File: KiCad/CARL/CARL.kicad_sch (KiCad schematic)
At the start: 39 parts, among them J1 Barrel_Jack (5V DC Supply), J2 SD_Card_Device, U1 NHD-0420H1Z (LCD), U2 LM386, U3 Led Driver

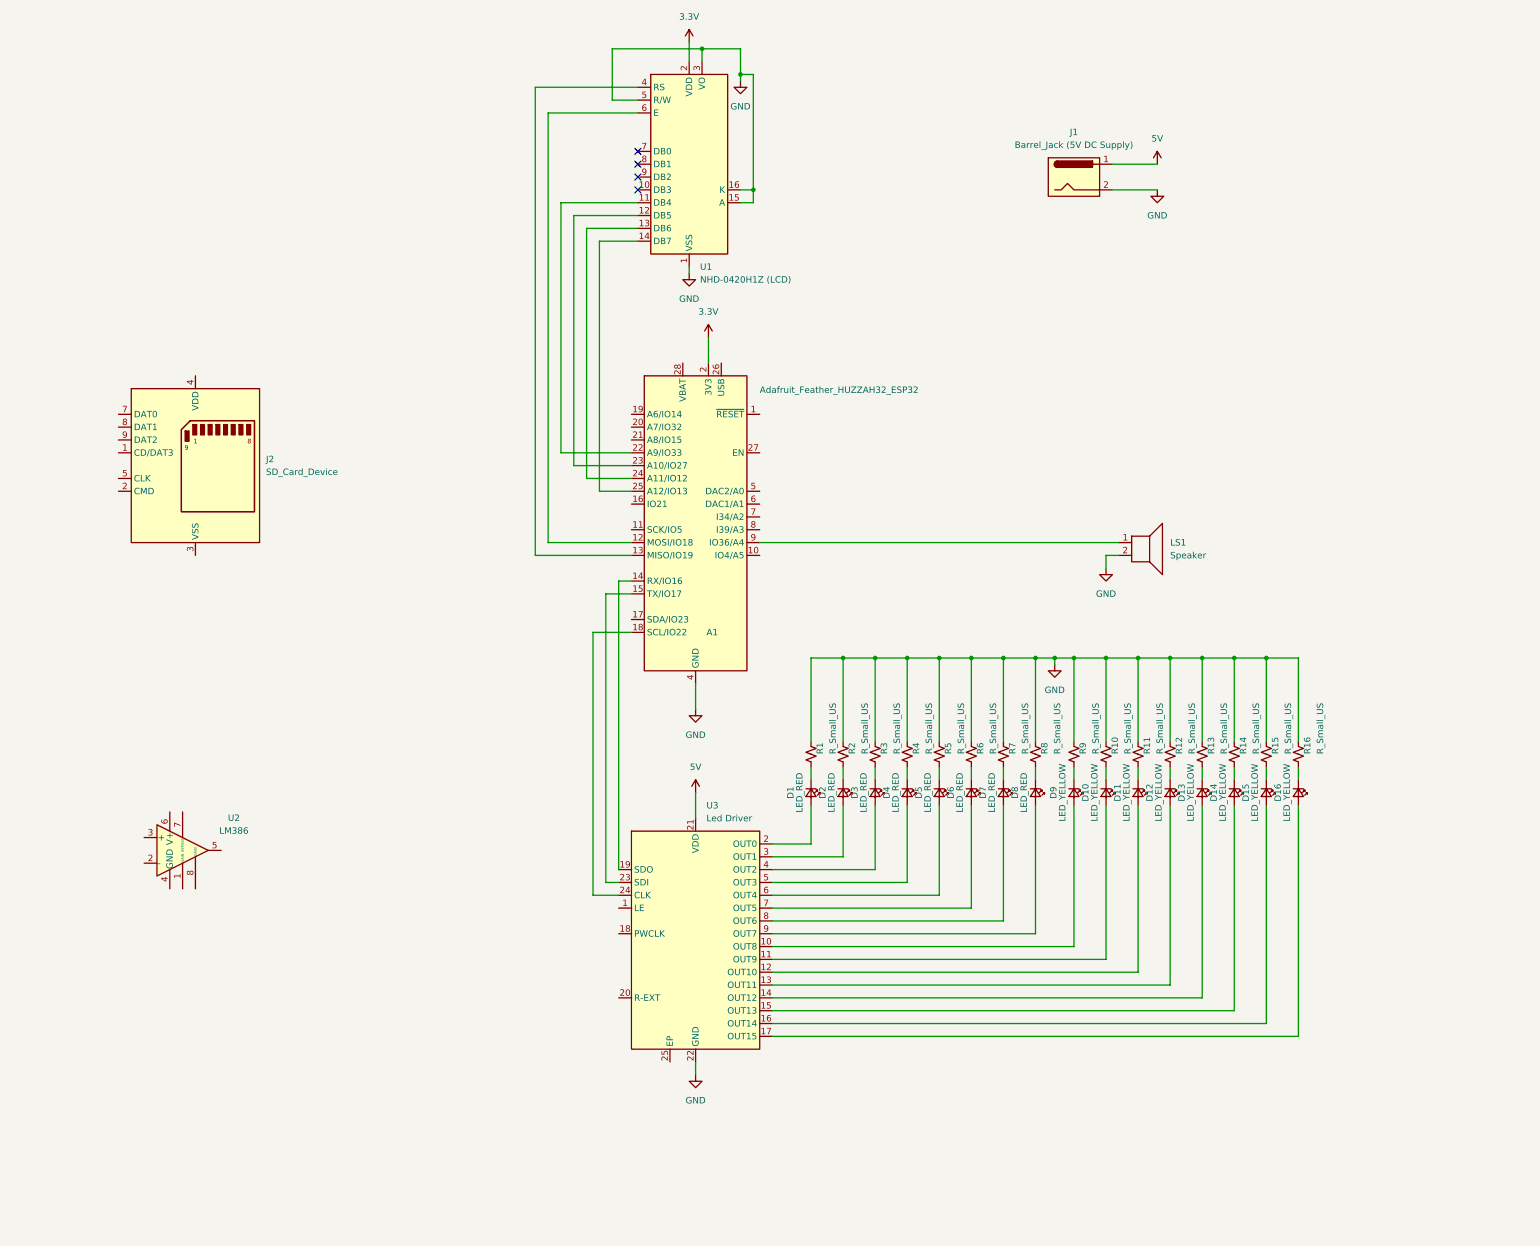
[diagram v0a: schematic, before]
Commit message: Update CARL.kicad_sch
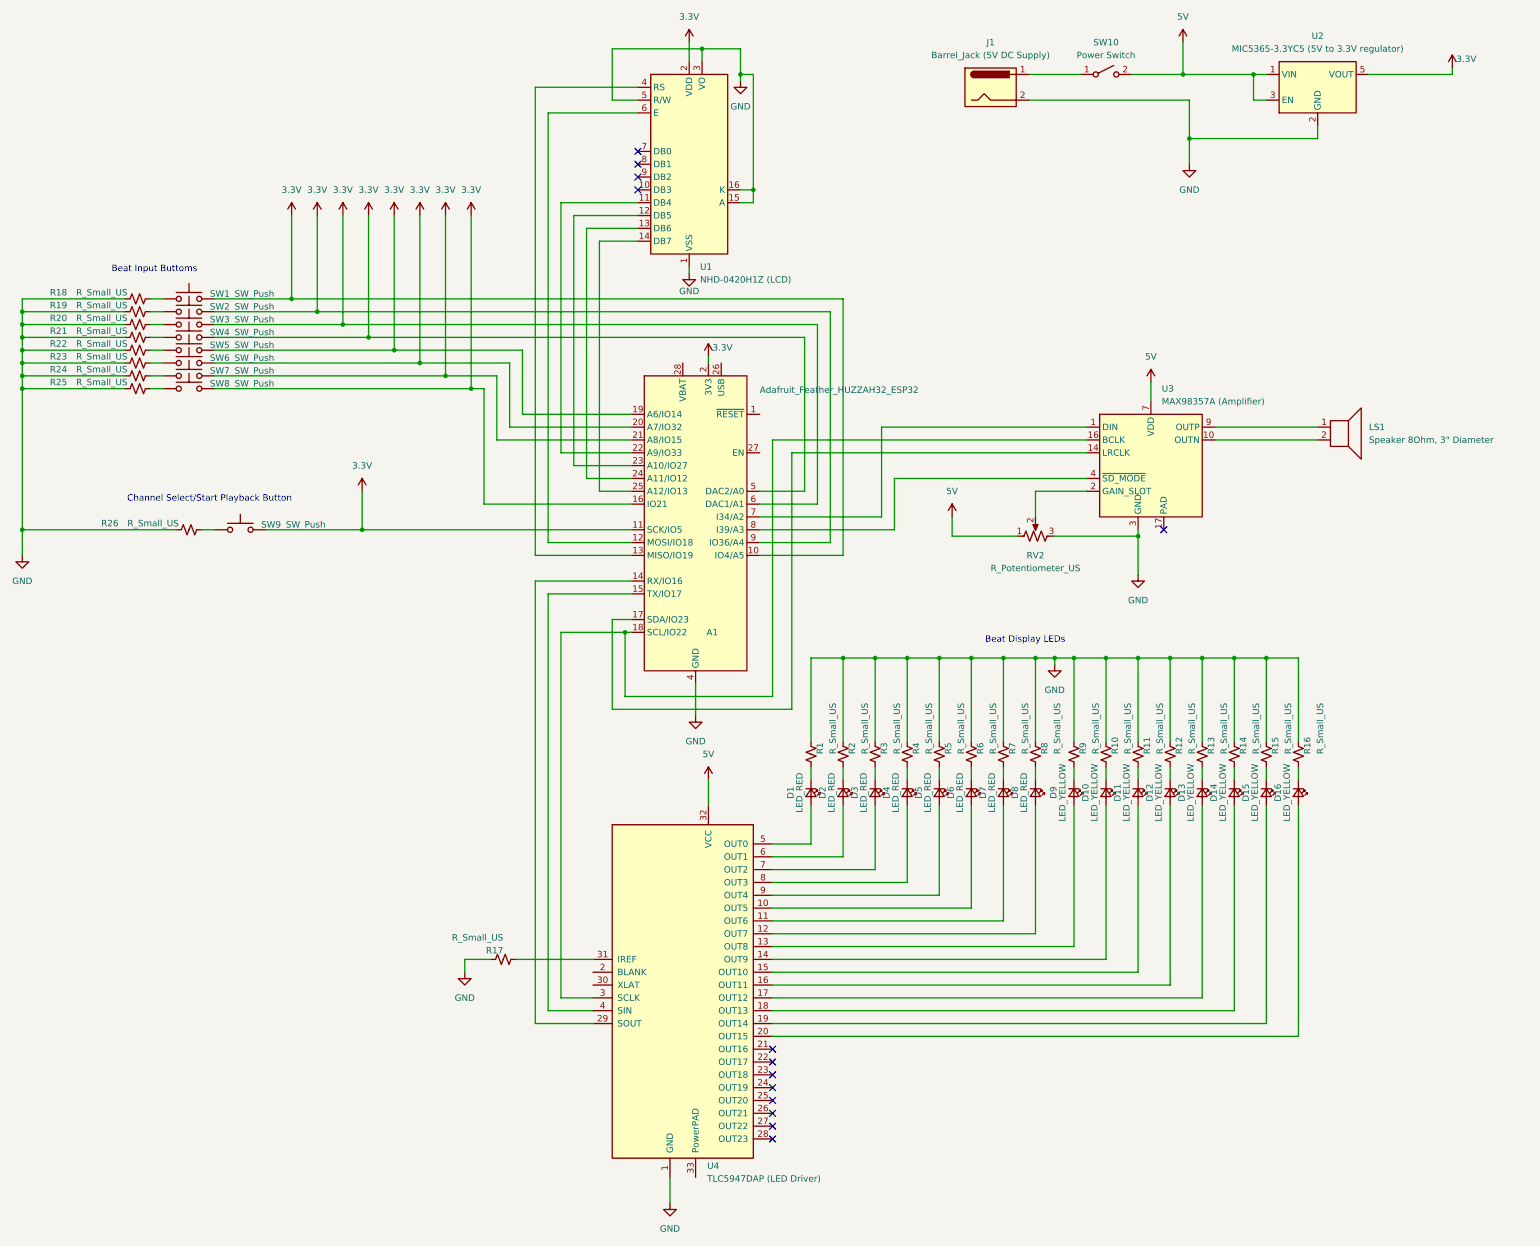
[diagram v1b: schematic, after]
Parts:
- removed J2: SD_Card_Device, symbol Connector:SD_Card_Device
- removed U2: LM386, symbol Amplifier_Audio:LM386
- removed U3: Led Driver, Package_DFN_QFN:QFN-24-1EP_4x4mm_P0.5mm_EP2.15x2.15mm, symbol Driver_LED:LED1642GWQTR
- added R17, R18, R19, R20, R21, R22, R23, R24, R25, R26: R_Small_US, symbol Device:R_Small_US
- added RV2: R_Potentiometer_US, symbol Device:R_Potentiometer_US
- added SW1, SW2, SW3, SW4, SW5, SW6, SW7, SW8, SW9: SW_Push, symbol Switch:SW_Push
- added SW10: Power Switch, symbol Switch:SW_SPST
- added U2: MIC5365-3.3YC5 (5V to 3.3V regulator), Package_TO_SOT_SMD:SOT-353_SC-70-5, symbol Regulator_Linear:MIC5365-3.3YC5
- added U3: MAX98357A (Amplifier), Package_DFN_QFN:TQFN-16-1EP_3x3mm_P0.5mm_EP1.23x1.23mm, symbol Audio:MAX98357A
- added U4: TLC5947DAP (LED Driver), Package_SO:HTSSOP-32-1EP_6.1x11mm_P0.65mm_EP5.2x11mm_Mask4.11x4.36mm_ThermalVias, symbol Driver_LED:TLC5947DAP
- LS1: value Speaker -> Speaker 8Ohm, 3" Diameter
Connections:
- net 3.3V: now also A1.10 (IO4/A5), A1.11 (SCK/IO5), A1.16 (IO21), A1.19 (A6/IO14), A1.20 (A7/IO32), A1.21 (A8/IO15), A1.5 (DAC2/A0), A1.6 (DAC1/A1), A1.9 (IO36/A4), SW1.2, SW2.2, SW3.2, SW4.2, SW5.2, SW6.2, SW7.2, SW8.2, SW9.2, U2.5 (VOUT)
- net 5V: now also RV2.1, SW10.2 (B), U2.1 (VIN), U2.3 (EN), U3.7 (VDD), U3.8 (VDD), U4.32 (VCC); no longer J1.1
- net GND: now also R17.1, R18.1, R19.1, R20.1, R21.1, R22.1, R23.1, R24.1, R25.1, R26.1, RV2.3, U2.2 (GND), U3.11 (GND), U3.15 (GND), U3.3 (GND), U4.1 (GND); no longer LS1.2
- net at D13.2 (A): now also U4.17 (OUT12)
- net at A1.14 (RX/IO16): now also U4.29 (SOUT)
- net at A1.15 (TX/IO17): now also U4.4 (SIN)
- net at A1.17 (SDA/IO23): now also U3.14 (LRCLK)
- net at A1.18 (SCL/IO22): now also U3.16 (BCLK), U4.3 (SCLK)
- net at A1.7 (I34/A2): now also U3.1 (DIN)
- net at A1.8 (I39/A3): now also U3.4 (~{SD_MODE})
- net at LS1.1: now also U3.9 (OUTP); no longer A1.9 (IO36/A4)
- net at D4.2 (A): now also U4.8 (OUT3)
- net at D14.2 (A): now also U4.18 (OUT13)
- net at D9.2 (A): now also U4.13 (OUT8)
- net at D10.2 (A): now also U4.14 (OUT9)
- net at D11.2 (A): now also U4.15 (OUT10)
- net at D12.2 (A): now also U4.16 (OUT11)
- net at D15.2 (A): now also U4.19 (OUT14)
- net at D16.2 (A): now also U4.20 (OUT15)
- net at D1.2 (A): now also U4.5 (OUT0)
- net at D2.2 (A): now also U4.6 (OUT1)
- net at D3.2 (A): now also U4.7 (OUT2)
- net at D5.2 (A): now also U4.9 (OUT4)
- net at D6.2 (A): now also U4.10 (OUT5)
- net at D7.2 (A): now also U4.11 (OUT6)
- net at D8.2 (A): now also U4.12 (OUT7)
- new net: R26.2, SW9.1
- new net: LS1.2, U3.10 (OUTN)
- new net: RV2.2, U3.2 (GAIN_SLOT)
- new net: R25.2, SW8.1
- new net: R21.2, SW4.1
- new net: R20.2, SW3.1
- new net: R23.2, SW6.1
- new net: J1.1, SW10.1 (A)
- new net: R18.2, SW1.1
- new net: R22.2, SW5.1
- new net: R19.2, SW2.1
- new net: R24.2, SW7.1
- new net: R17.2, U4.31 (IREF)
- no-connect marks 4 -> 13
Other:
- note added: "Beat Display LEDs"
- note added: "Beat Input Buttoms"
- note added: "Channel Select/Start Playback Button"
- moved on the sheet: J1, LS1
